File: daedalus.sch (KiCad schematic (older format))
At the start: 101 parts, among them J1 CAN Bus, J2 CAN Bus, J3 I2C 1 Breakout, J4 I2C 1 Breakout, J5 A Terminal, J6 B Terminal, J7 C Terminal, J8 SWD, J9 USB_B_Micro, Q1 AO3401A, U1 XT30, U10 TPH, U11 TPH, U12 TPH, U13 TPH, U14 USBLC6-2SC6, U2 XT30, U3 MP2359DJ-LF-Z, U4 MA700, U5 DRV8323RH, U6 MCP2542, U7 STM32F405RGTx, U8 TPH, U9 TPH, Y1 16MHz

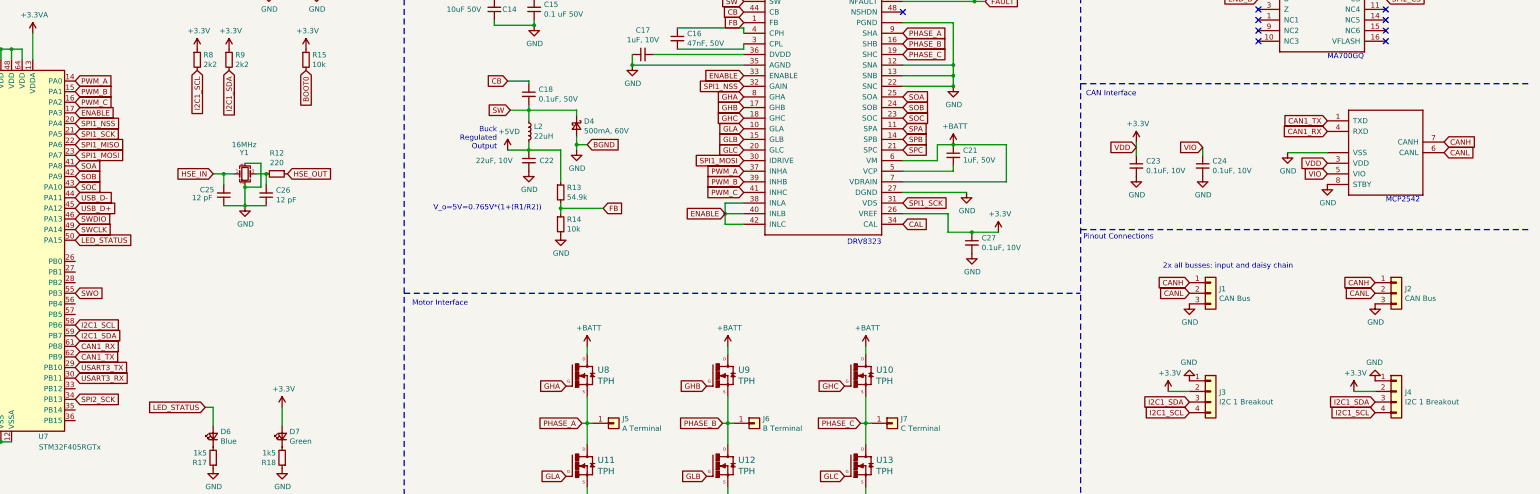
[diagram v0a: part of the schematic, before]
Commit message: Updated footprint and routing
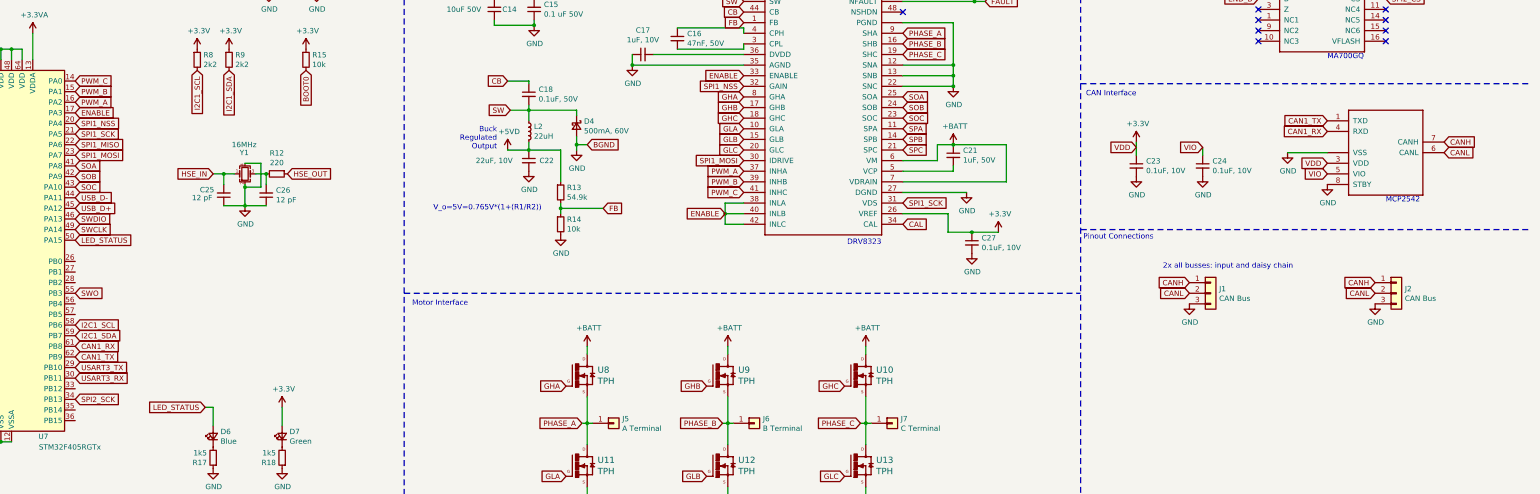
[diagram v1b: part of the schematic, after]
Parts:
- removed J3, J4: I2C 1 Breakout, Connector_JST:JST_PH_S4B-PH-K_1x04_P2.00mm_Horizontal, symbol Connector_Generic:Conn_01x04
- J1, J2: footprint Connector_JST:JST_PH_S3B-PH-K_1x03_P2.00mm_Horizontal -> Connector_JST:JST_PH_S3B-PH-SM4-TB_1x03-1MP_P2.00mm_Horizontal
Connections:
- net PWM_A: now also U7.16 (PA2); no longer U7.14 (PA0)
- net PWM_C: now also U7.14 (PA0); no longer U7.16 (PA2)
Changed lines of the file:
@@
 Text Notes 9800 575  0    50   ~ 0
 Power and Mounting Points
-$Comp
-L Connector_Generic:Conn_01x04 J3
-U 1 1 6033D355
-P 13500 6600
-F 0 "J3" H 13580 6592 50  0000 L CNN
-F 1 "I2C 1 Breakout" H 13580 6501 50  0000 L CNN
-F 2 "Connector_JST:JST_PH_S4B-PH-K_1x04_P2.00mm_Horizontal" H 13500 6600 50  0001 C CNN
-F 3 "~" H 13500 6600 50  0001 C CNN
-	1    13500 6600
-	1    0    0    -1
-$EndComp
-Text GLabel 13300 6700 0    50   Input ~ 0
-I2C1_SDA
-Text GLabel 13300 6800 0    50   Input ~ 0
-I2C1_SCL
-$Comp
-L power:GND #PWR061
-U 1 1 60342267
-P 13300 6500
-F 0 "#PWR061" H 13300 6250 50  0001 C CNN
-F 1 "GND" H 13305 6327 50  0000 C CNN
-F 2 "" H 13300 6500 50  0001 C CNN
-F 3 "" H 13300 6500 50  0001 C CNN
-	1    13300 6500
-	-1   0    0    1
-$EndComp
-$Comp
-L power:+3.3V #PWR063
-U 1 1 60343CEB
-P 13100 6600
-F 0 "#PWR063" H 13100 6450 50  0001 C CNN
-F 1 "+3.3V" H 13115 6773 50  0000 C CNN
-F 2 "" H 13100 6600 50  0001 C CNN
-F 3 "" H 13100 6600 50  0001 C CNN
-	1    13100 6600
-	1    0    0    -1
-$EndComp
-Wire Wire Line
-	13100 6600 13300 6600
 Text GLabel 2800 4175 2    50   Input ~ 0
 SPI1_SCK
@@
 Text GLabel 2800 6675 2    50   Input ~ 0
 SPI2_SCK
-Text GLabel 2800 3675 2    50   Input ~ 0
+Text GLabel 2800 3875 2    50   Input ~ 0
 PWM_A
 Text GLabel 2800 3775 2    50   Input ~ 0
 PWM_B
-Text GLabel 2800 3875 2    50   Input ~ 0
+Text GLabel 2800 3675 2    50   Input ~ 0
 PWM_C
 Text GLabel 2800 3975 2    50   Input ~ 0
@@
 F 0 "J1" H 13580 5717 50  0000 L CNN
 F 1 "CAN Bus" H 13580 5626 50  0000 L CNN
-F 2 "Connector_JST:JST_PH_S3B-PH-K_1x03_P2.00mm_Horizontal" H 13500 5675 50  0001 C CNN
+F 2 "Connector_JST:JST_PH_S3B-PH-SM4-TB_1x03-1MP_P2.00mm_Horizontal" H 13500 5675 50  0001 C CNN
 F 3 "~" H 13500 5675 50  0001 C CNN
 	1    13500 5675
@@
 F 0 "J2" H 15330 5717 50  0000 L CNN
 F 1 "CAN Bus" H 15330 5626 50  0000 L CNN
-F 2 "Connector_JST:JST_PH_S3B-PH-K_1x03_P2.00mm_Horizontal" H 15250 5675 50  0001 C CNN
+F 2 "Connector_JST:JST_PH_S3B-PH-SM4-TB_1x03-1MP_P2.00mm_Horizontal" H 15250 5675 50  0001 C CNN
 F 3 "~" H 15250 5675 50  0001 C CNN
 	1    15250 5675
@@
 Text Notes 12475 1825 0    50   ~ 0
 Two XT30 plugs: power in and daisy chaining
-$Comp
-L Connector_Generic:Conn_01x04 J4
-U 1 1 603C1235
-P 15250 6600
-F 0 "J4" H 15330 6592 50  0000 L CNN
-F 1 "I2C 1 Breakout" H 15330 6501 50  0000 L CNN
-F 2 "Connector_JST:JST_PH_S4B-PH-K_1x04_P2.00mm_Horizontal" H 15250 6600 50  0001 C CNN
-F 3 "~" H 15250 6600 50  0001 C CNN
-	1    15250 6600
-	1    0    0    -1
-$EndComp
-Text GLabel 15050 6700 0    50   Input ~ 0
-I2C1_SDA
-Text GLabel 15050 6800 0    50   Input ~ 0
-I2C1_SCL
-$Comp
-L power:GND #PWR062
-U 1 1 603C123D
-P 15050 6500
-F 0 "#PWR062" H 15050 6250 50  0001 C CNN
-F 1 "GND" H 15055 6327 50  0000 C CNN
-F 2 "" H 15050 6500 50  0001 C CNN
-F 3 "" H 15050 6500 50  0001 C CNN
-	1    15050 6500
-	-1   0    0    1
-$EndComp
-$Comp
-L power:+3.3V #PWR064
-U 1 1 603C1243
-P 14850 6600
-F 0 "#PWR064" H 14850 6450 50  0001 C CNN
-F 1 "+3.3V" H 14865 6773 50  0000 C CNN
-F 2 "" H 14850 6600 50  0001 C CNN
-F 3 "" H 14850 6600 50  0001 C CNN
-	1    14850 6600
-	1    0    0    -1
-$EndComp
-Wire Wire Line
-	14850 6600 15050 6600
 Text Notes 13050 5450 0    50   ~ 0
 2x all busses: input and daisy chain
